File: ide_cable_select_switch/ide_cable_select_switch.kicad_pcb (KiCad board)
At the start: 2 copper layers, 23.9 x 56.9 mm, 4 parts, among them J1 Conn_02x20_Odd_Even, J2 Conn_02x20_Odd_Even, J3 Conn_02x20_Odd_Even, SW1 SW_SPDT

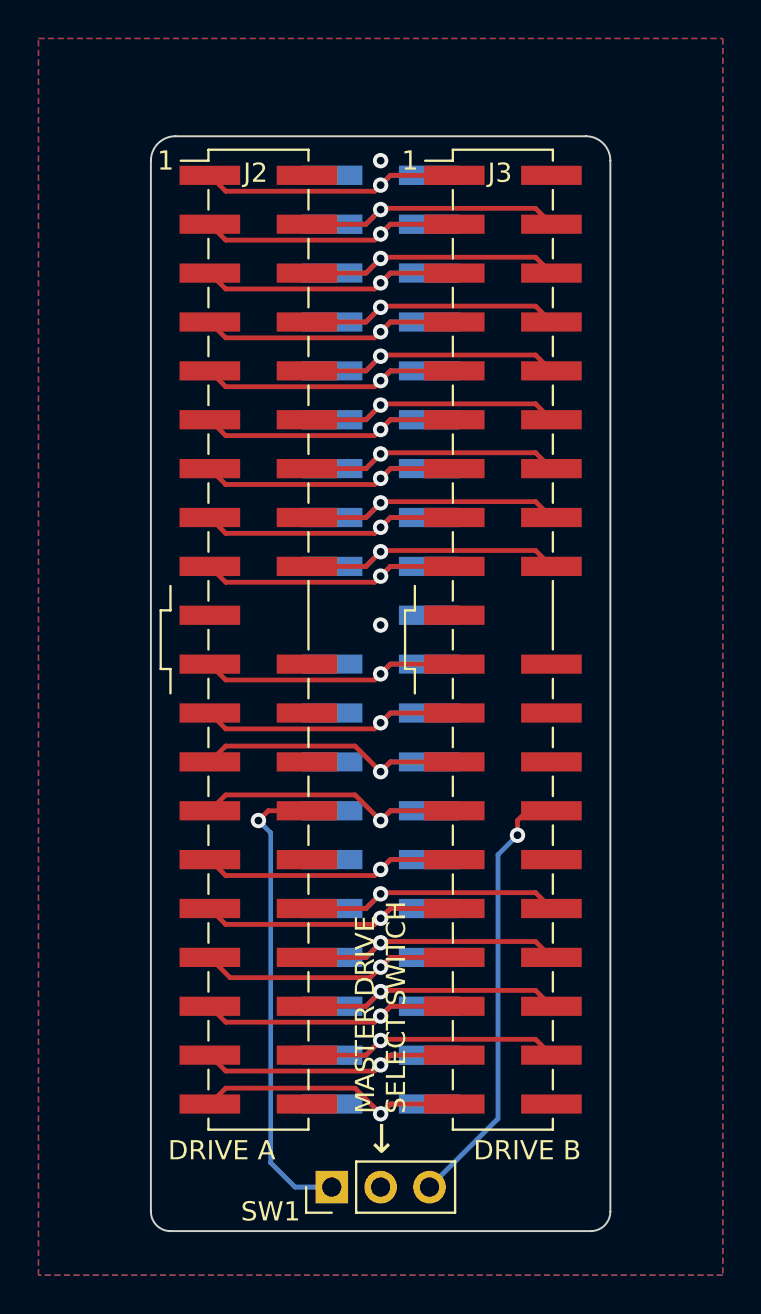
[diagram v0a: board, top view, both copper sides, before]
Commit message: previous fab changes
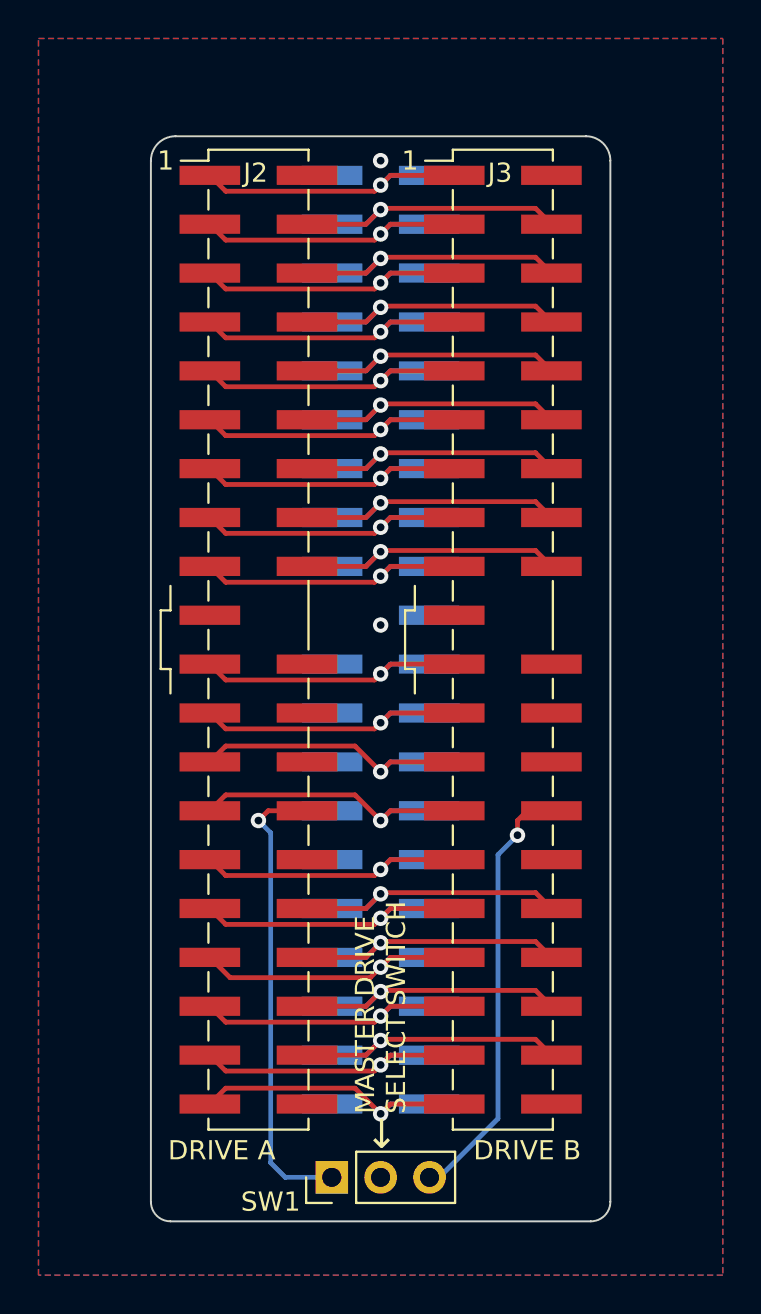
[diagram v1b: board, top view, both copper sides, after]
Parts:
- moved SW1 0.51 mm to (152.4, 112.5)
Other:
- board size 23.9 x 56.9 mm -> 23.9 x 56.4 mm
- board text added: "IDE DRIVE CABLE SELECT SWITCH"
- board text removed: "IDE DRIVE CABLE SELECT SWITCHER"
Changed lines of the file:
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@@
   (net 35 "CSEL_OUT_B")
   (footprint "Connector_PinHeader_2.54mm:PinHeader_1x03_P2.54mm_Vertical" (layer "F.Cu")
-    (at 152.4 113.03 90)
+    (at 152.4 112.522 90)
     (descr "Through hole straight pin header, 1x03, 2.54mm pitch, single row")
     (tags "Through hole pin header THT 1x03 2.54mm single row")
@@
     )
   )
-  (gr_line (start 166.878 114.3) (end 166.878 59.69) (layer "Edge.Cuts") (width 0.1))
+  (gr_line (start 166.878 113.792) (end 166.878 59.69) (layer "Edge.Cuts") (width 0.1))
   (gr_line (start 165.608 58.42) (end 144.272 58.42) (layer "Edge.Cuts") (width 0.1))
-  (gr_line (start 144.018 115.316) (end 165.862 115.316) (layer "Edge.Cuts") (width 0.1))
-  (gr_arc (start 144.018 115.316) (mid 143.29958 115.01842) (end 143.002001 114.3) (layer "Edge.Cuts") (width 0.1))
-  (gr_arc (start 166.878 114.3) (mid 166.58042 115.01842) (end 165.862 115.316) (layer "Edge.Cuts") (width 0.1))
+  (gr_line (start 144.018 114.808) (end 165.862 114.808) (layer "Edge.Cuts") (width 0.1))
+  (gr_arc (start 144.018 114.808) (mid 143.29958 114.51042) (end 143.002001 113.792) (layer "Edge.Cuts") (width 0.1))
+  (gr_arc (start 166.878 113.792) (mid 166.58042 114.51042) (end 165.862 114.808) (layer "Edge.Cuts") (width 0.1))
   (gr_arc (start 165.608 58.42) (mid 166.506026 58.791974) (end 166.878 59.69) (layer "Edge.Cuts") (width 0.1))
   (gr_arc (start 143.002 59.69) (mid 143.373974 58.791974) (end 144.272 58.42) (layer "Edge.Cuts") (width 0.1))
-  (gr_line (start 143.002 59.69) (end 143.002001 114.3) (layer "Edge.Cuts") (width 0.1))
+  (gr_line (start 143.002 59.69) (end 143.002001 113.792) (layer "Edge.Cuts") (width 0.1))
   (gr_text "github.com/xunker ©2022\nCC NC-BY-SA 4.0" (at 163.195 71.755 90) (layer "B.SilkS")
     (effects (font (size 1 1) (thickness 0.15)) (justify mirror))
@@
     (effects (font (size 0.9 0.9) (thickness 0.15)) (justify right mirror))
   )
-  (gr_text "IDE DRIVE CABLE SELECT SWITCHER" (at 144.78 102.87 90) (layer "B.SilkS")
-    (effects (font (size 1.25 1.25) (thickness 0.15)) (justify right mirror))
-  )
-  (gr_text "‼" (at 147.955 113.03 90) (layer "B.SilkS")
+  (gr_text "IDE DRIVE CABLE SELECT SWITCH" (at 144.78 85.09 90) (layer "B.SilkS")
+    (effects (font (size 1.25 1.25) (thickness 0.15)) (justify mirror))
+  )
+  (gr_text "‼" (at 147.955 111.252 90) (layer "B.SilkS")
     (effects (font (size 1.75 1.75) (thickness 0.3)) (justify mirror))
   )
-  (gr_text "Change Master Drive Select Switch\nONLY while system power is OFF" (at 147.955 99.06 90) (layer "B.SilkS")
+  (gr_text "Change Master Drive Select Switch\nONLY while system power is OFF" (at 148.336 98.044 90) (layer "B.SilkS")
     (effects (font (size 0.9 0.9) (thickness 0.15)) (justify mirror))
   )
@@
     (effects (font (size 1 1) (thickness 0.15)) (justify mirror))
   )
-  (gr_text "‼" (at 147.955 85.09 90) (layer "B.SilkS")
+  (gr_text "‼" (at 147.955 84.836 90) (layer "B.SilkS")
     (effects (font (size 1.75 1.75) (thickness 0.3)) (justify mirror))
   )
@@
     (effects (font (size 1 1) (thickness 0.15)))
   )
-  (gr_text "←" (at 154.94 110.49 90) (layer "F.SilkS")
+  (gr_text "←" (at 154.94 110.236 90) (layer "F.SilkS")
     (effects (font (size 1.5 1.5) (thickness 0.15)))
   )
@@
   )
   (dimension (type aligned) (layer "Dwgs.User")
-    (pts (xy 166.878 58.801) (xy 166.878 115.316))
+    (pts (xy 166.878 58.801) (xy 166.878 114.808))
     (height -5.08)
-    (gr_text "56.5150 mm" (at 170.808 87.0585 90) (layer "Dwgs.User")
+    (gr_text "56.0070 mm" (at 170.808 86.8045 90) (layer "Dwgs.User")
       (effects (font (size 1 1) (thickness 0.15)))
     )
@@
   (segment (start 148.59 93.98) (end 149.098 93.472) (width 0.25) (layer "F.Cu") (net 34))
   (via (at 148.59 93.98) (size 0.8) (drill 0.4) (layers "F.Cu" "B.Cu") (net 34))
-  (segment (start 150.495 113.03) (end 152.4 113.03) (width 0.25) (layer "B.Cu") (net 34))
+  (segment (start 149.987 112.522) (end 152.4 112.522) (width 0.25) (layer "B.Cu") (net 34))
+  (segment (start 148.59 93.98) (end 149.225 94.615) (width 0.25) (layer "B.Cu") (net 34))
+  (segment (start 149.225 111.76) (end 149.987 112.522) (width 0.25) (layer "B.Cu") (net 34))
   (segment (start 149.225 94.615) (end 149.225 111.76) (width 0.25) (layer "B.Cu") (net 34))
-  (segment (start 149.225 111.76) (end 150.495 113.03) (width 0.25) (layer "B.Cu") (net 34))
-  (segment (start 148.59 93.98) (end 149.225 94.615) (width 0.25) (layer "B.Cu") (net 34))
   (segment (start 162.052 93.98) (end 162.56 93.472) (width 0.25) (layer "F.Cu") (net 35))
   (segment (start 162.052 94.742) (end 162.052 93.98) (width 0.25) (layer "F.Cu") (net 35))
   (segment (start 162.56 93.472) (end 163.815 93.472) (width 0.25) (layer "F.Cu") (net 35))
   (via (at 162.052 94.742) (size 0.8) (drill 0.4) (layers "F.Cu" "B.Cu") (net 35))
+  (segment (start 161.036 109.474) (end 157.988 112.522) (width 0.25) (layer "B.Cu") (net 35))
+  (segment (start 162.052 94.742) (end 161.036 95.758) (width 0.25) (layer "B.Cu") (net 35))
+  (segment (start 157.988 112.522) (end 157.48 112.522) (width 0.25) (layer "B.Cu") (net 35))
   (segment (start 161.036 95.758) (end 161.036 109.474) (width 0.25) (layer "B.Cu") (net 35))
-  (segment (start 161.036 109.474) (end 157.48 113.03) (width 0.25) (layer "B.Cu") (net 35))
-  (segment (start 162.052 94.742) (end 161.036 95.758) (width 0.25) (layer "B.Cu") (net 35))
   (zone (net 2) (net_name "GND") (layers F&B.Cu) (hatch edge 0.508)
     (connect_pads (clearance 0.508))
